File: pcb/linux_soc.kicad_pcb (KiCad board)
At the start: 2 copper layers, 25.5 x 32 mm, 60 parts, among them J2 USB_C_Receptacle_USB2.0_16P, J3 Micro_SD_Card, U1 F1C100s, U2 TMI7003C, Y1 24MHz

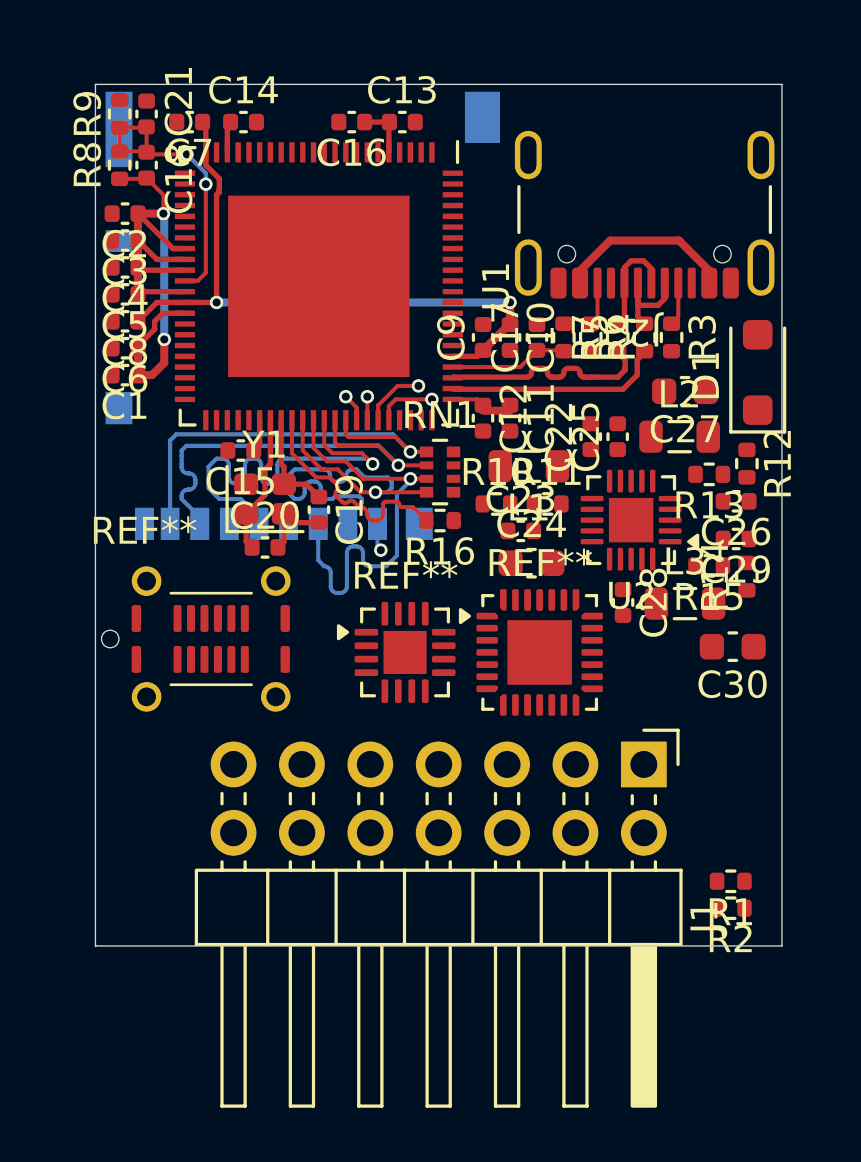
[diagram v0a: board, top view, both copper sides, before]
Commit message: Completed PCB
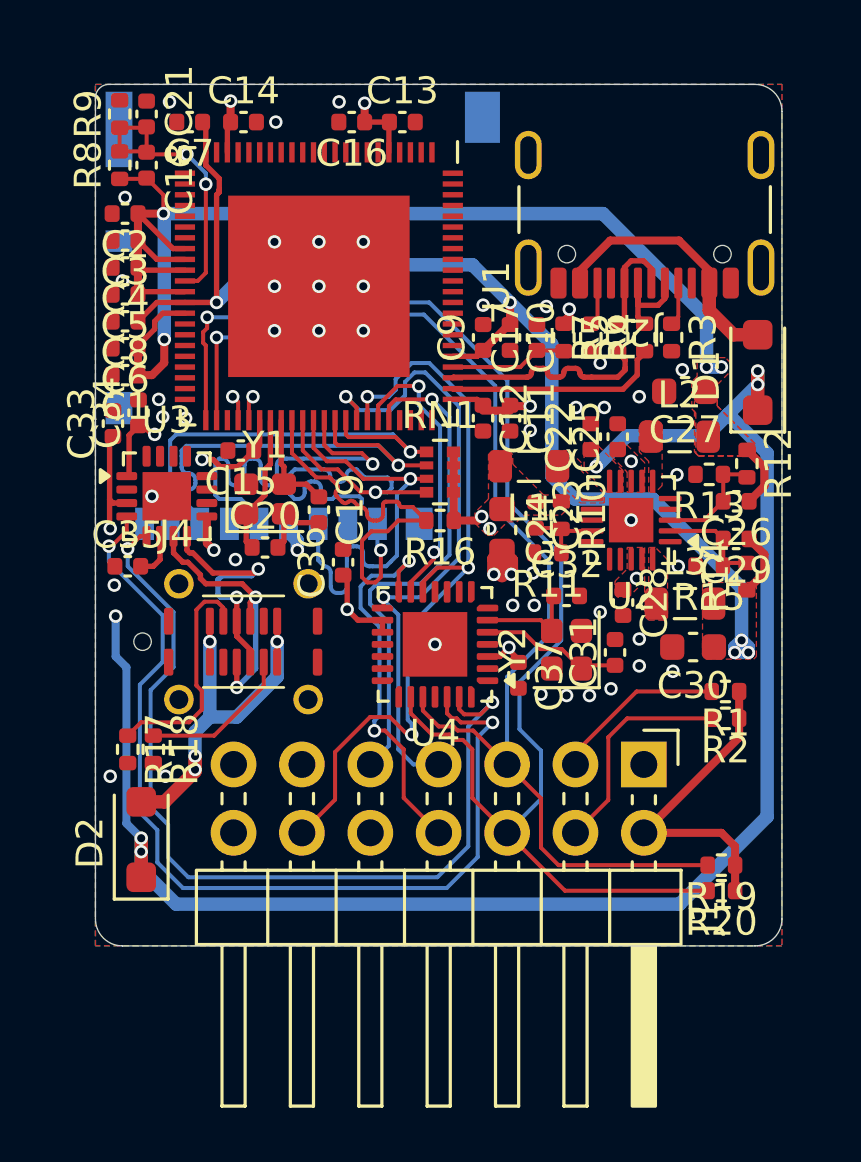
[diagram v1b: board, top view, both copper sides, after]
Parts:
- removed REF**: TQFN-16-1EP_3x3mm_P0.5mm_EP1.6x1.6mm, Package_DFN_QFN:TQFN-16-1EP_3x3mm_P0.5mm_EP1.6x1.6mm
- removed REF**: QFN-28-1EP_4x4mm_P0.45mm_EP2.4x2.4mm, Package_DFN_QFN:QFN-28-1EP_4x4mm_P0.45mm_EP2.4x2.4mm
- removed REF**: USB_C_Receptacle_Vertical, linux_soc:USB_C_Receptacle_Vertical
- added C31: C, Capacitor_SMD:C_0402_1005Metric, F.Cu at (119.3, 121.1)
- added C32: C, Capacitor_SMD:C_0402_1005Metric, F.Cu at (117.5, 119.0)
- added C33: 100n, Capacitor_SMD:C_0402_1005Metric, F.Cu at (100.7, 112.6)
- added C34: 100n, Capacitor_SMD:C_0402_1005Metric, F.Cu at (101.6, 112.2)
- added C35: 100n, Capacitor_SMD:C_0402_1005Metric, F.Cu at (101.2, 117.9)
- added C36: 100n, Capacitor_SMD:C_0402_1005Metric, F.Cu at (109.2, 117.8)
- added C37: 100n, Capacitor_SMD:C_0402_1005Metric, F.Cu at (115.7, 122.0)
- added D2: DSK24L, Diode_SMD:D_SOD-123F, F.Cu at (101.7, 128.1)
- added J4: USB_C_Receptacle_USB2.0_16P, linux_soc:USB_C_Receptacle_Vertical, F.Cu at (105.5, 120.7)
- added R17: 5k1, Resistor_SMD:R_0402_1005Metric, F.Cu at (101.2, 124.7)
- added R18: 5k1, Resistor_SMD:R_0402_1005Metric, F.Cu at (102.2, 124.7)
- added R19: 4k7, Resistor_SMD:R_0402_1005Metric, F.Cu at (123.2, 129.0)
- added R20: 4k7, Resistor_SMD:R_0402_1005Metric, F.Cu at (123.2, 129.9)
- added U3: CH343P, Package_DFN_QFN:WCH_QFN-16-1EP_3x3mm_P0.5mm_EP1.8x1.8mm, F.Cu at (102.7, 115.3)
- added U4: ATmega328P-MM, Package_DFN_QFN:QFN-28-1EP_4x4mm_P0.45mm_EP2.4x2.4mm, F.Cu at (112.6, 120.8)
- added Y2: 24MHz, Crystal:Crystal_SMD_2016-4Pin_2.0x1.6mm, F.Cu at (117.5, 121.0)
- moved R1 7.05 mm to (123.4, 122.5)
- moved R2 7.05 mm to (123.4, 123.5)
- moved R10 2.44 mm to (117.3, 116.0), turned to -90 degrees
- moved R11 1.81 mm to (116.8, 117.4), turned to 180 degrees
- moved C24 1.65 mm to (115.1, 116.5), turned to -90 degrees
- moved C30 1.47 mm to (122.2, 120.9)
- moved C23 0.80 mm to (116.3, 116.0), turned to -90 degrees
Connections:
- U1 pad 61: /SPI_MISO -> /SPI_DAISY
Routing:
- net +5V: track 0.00 -> 75.7 mm, vias 0 -> 8
- net /I2C_SDA: track 0.00 -> 51.1 mm, vias 0 -> 1
- net /I2C_SCL: track 0.00 -> 44.9 mm, vias 0 -> 1
- net /MICROCONTROLLER/TX: track 0.00 -> 35.1 mm, vias 0 -> 2
- net /MICROCONTROLLER/RX: track 0.00 -> 33.3 mm, vias 0 -> 2
- net +3V3: track 6.66 -> 36.2 mm, vias 0 -> 13
- net /SPI_CS: track 0.88 -> 28.8 mm, vias 1 -> 3
- net +2V5: track 24.7 -> 51.2 mm, vias 2 -> 4
- net +1V1: track 24.5 -> 47.5 mm, vias 2 -> 5
- net /SPI_SCK: track 1.04 -> 23.9 mm, vias 1 -> 2
- net /UART_TX: track 0.00 -> 20.2 mm, vias 0 -> 1
- net /SPI_MOSI: track 2.23 -> 18.8 mm
- net /UART_RX: track 0.00 -> 16.3 mm, vias 0 -> 1
- net Net-(D2-A): track 0.00 -> 15.5 mm, vias 0 -> 4
- net /SPI_MISO: track 2.35 -> 14.3 mm, vias 1 -> 2
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- added copper zone on F.Cu, net +1V1
- added copper zone on F.Cu, net +2V5
- added copper zone on F.Cu, net +3V3
- added copper zone on In2.Cu, net +3V3
- added copper zone on F.Cu, net +5V
- added copper zone on B.Cu, net GND
- added copper zone on F.Cu, net GND
- added copper zone on In1.Cu, net GND
- added copper zone on F.Cu, net Net-(U2-LX1)
- added copper zone on F.Cu, net Net-(U2-LX2)
- added copper zone on F.Cu, net Net-(U2-LX3)
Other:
- outline, holes or cut-outs redrawn
- copper layers 2 -> 4
